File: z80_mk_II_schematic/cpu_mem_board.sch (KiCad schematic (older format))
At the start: 23 parts

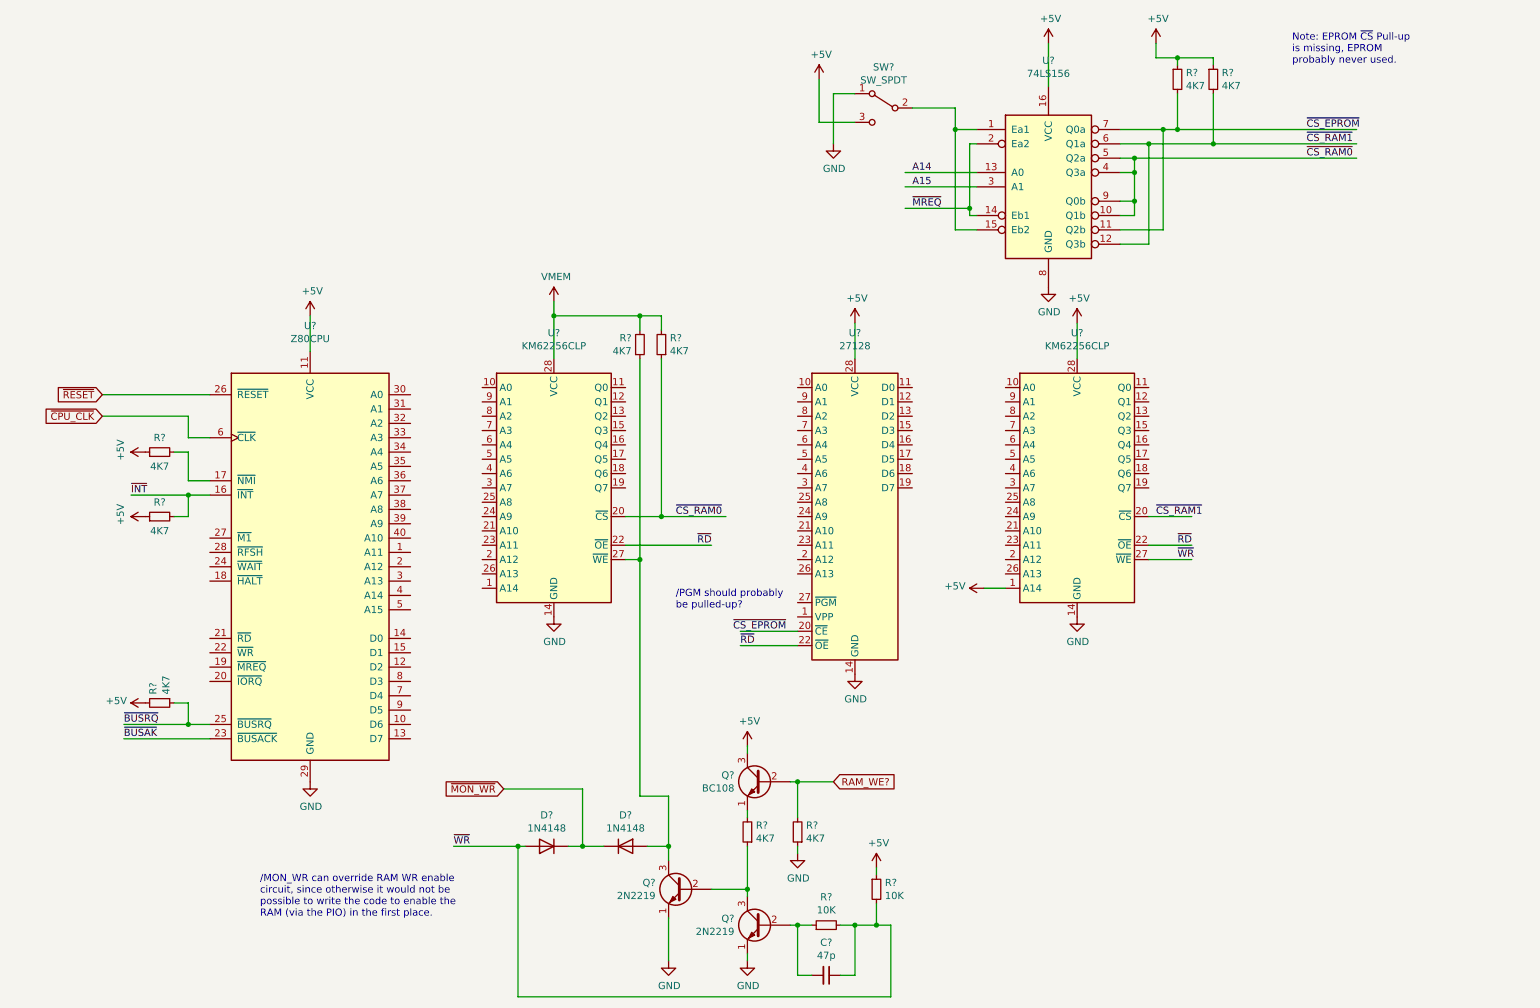
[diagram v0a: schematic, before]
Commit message: Lots more work on schematic
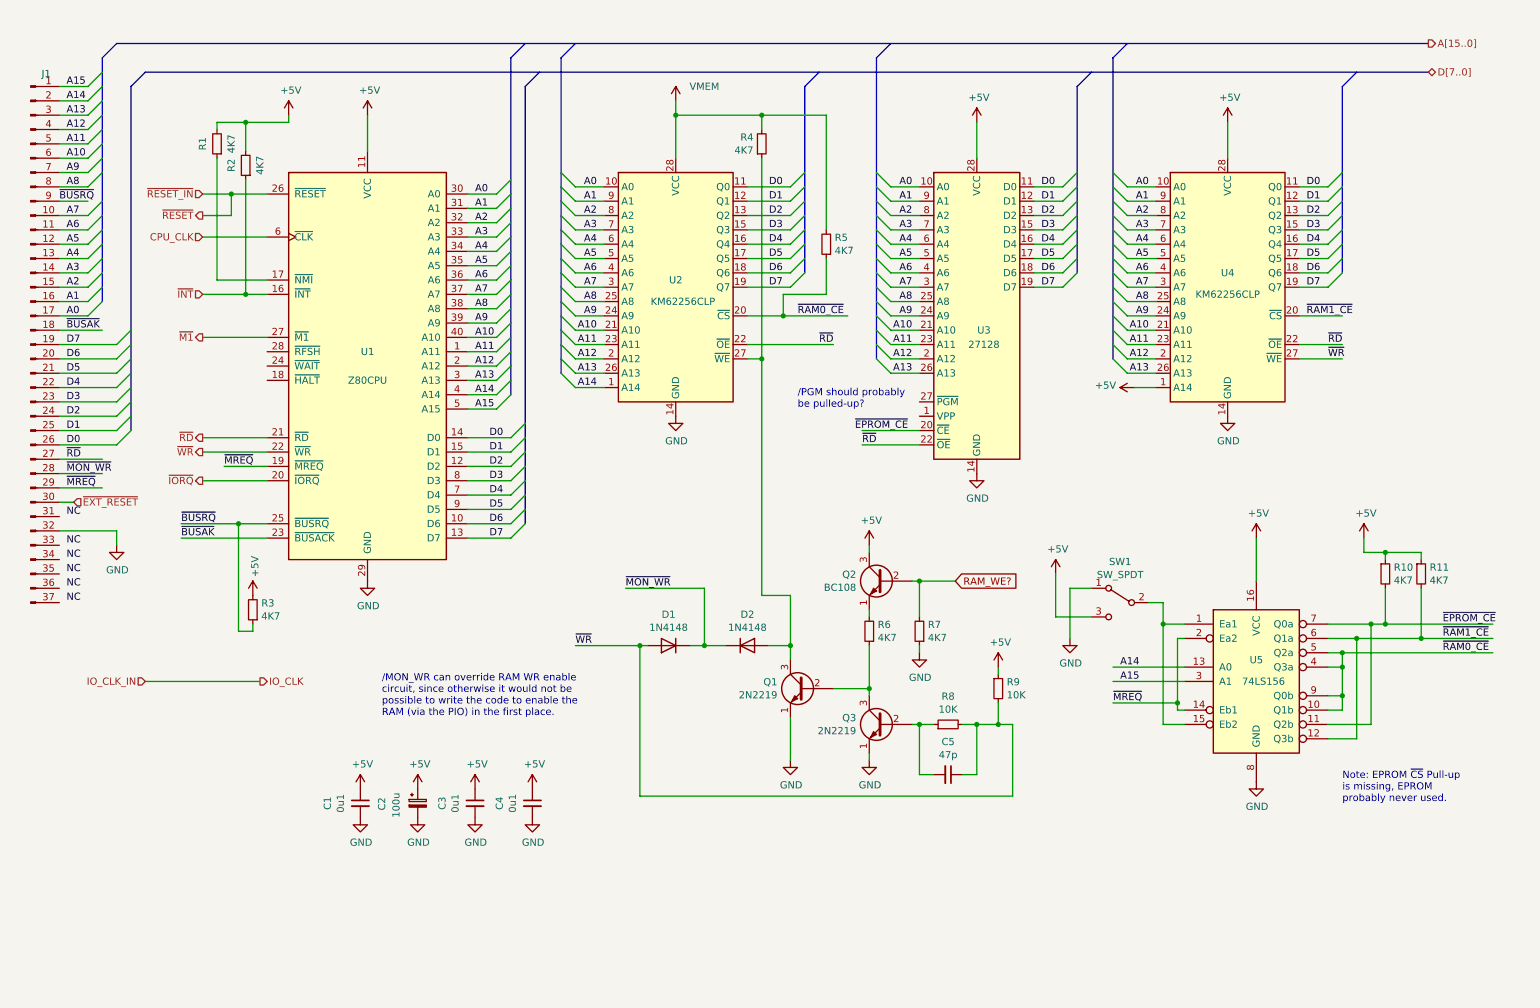
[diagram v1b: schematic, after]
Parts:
- added C1, C3, C4: 0u1, symbol Device:C_Small
- added C2: 100u, symbol Device:CP_Small
- added J1: Conn_01x37_Male, symbol Connector:Conn_01x37_Male
- gave numbers to parts that had none: 23
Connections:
- net labels added: A0, A1, A10, A11, A12, A13, A2, A3, A4, A5, A6, A7, A8, A9, A[15..0], CPU_CLK, D0, D1, D2, D3, D4, D5, D6, D7, D[7..0], IO_CLK, IO_CLK_IN, NC, ~BUSAK~, ~BUSRQ~, ~EPROM_CE~, ~EXT_RESET~, ~INT~, ~IORQ~, ~M1~, ~MON_WR~, ~MREQ~, ~RAM0_CE~, ~RAM1_CE~, ~RD~, ~RESET_IN~, ~RESET~, ~WR~
- net labels removed: ~BUSAK, ~BUSRQ, ~CPU_CLK, ~CS_EPROM, ~CS_RAM0, ~CS_RAM1, ~INT, ~MON_WR, ~MREQ, ~RD, ~RESET
- wire segments 115 -> 251
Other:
- moved on the sheet: C5, D1, D2, Q1, Q2, Q3, R1, R10, R11, R2, R3, R4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
